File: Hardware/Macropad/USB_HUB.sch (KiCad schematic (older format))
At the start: 25 parts, among them J4 USB_C_Receptacle_USB2.0, J5 USB_C_Receptacle_USB2.0, J6 USB_C_Receptacle_USB2.0, U4 TUSB2046b, U6 SRV05-4, U8 SRV05-4, X2 625L3C006M00000

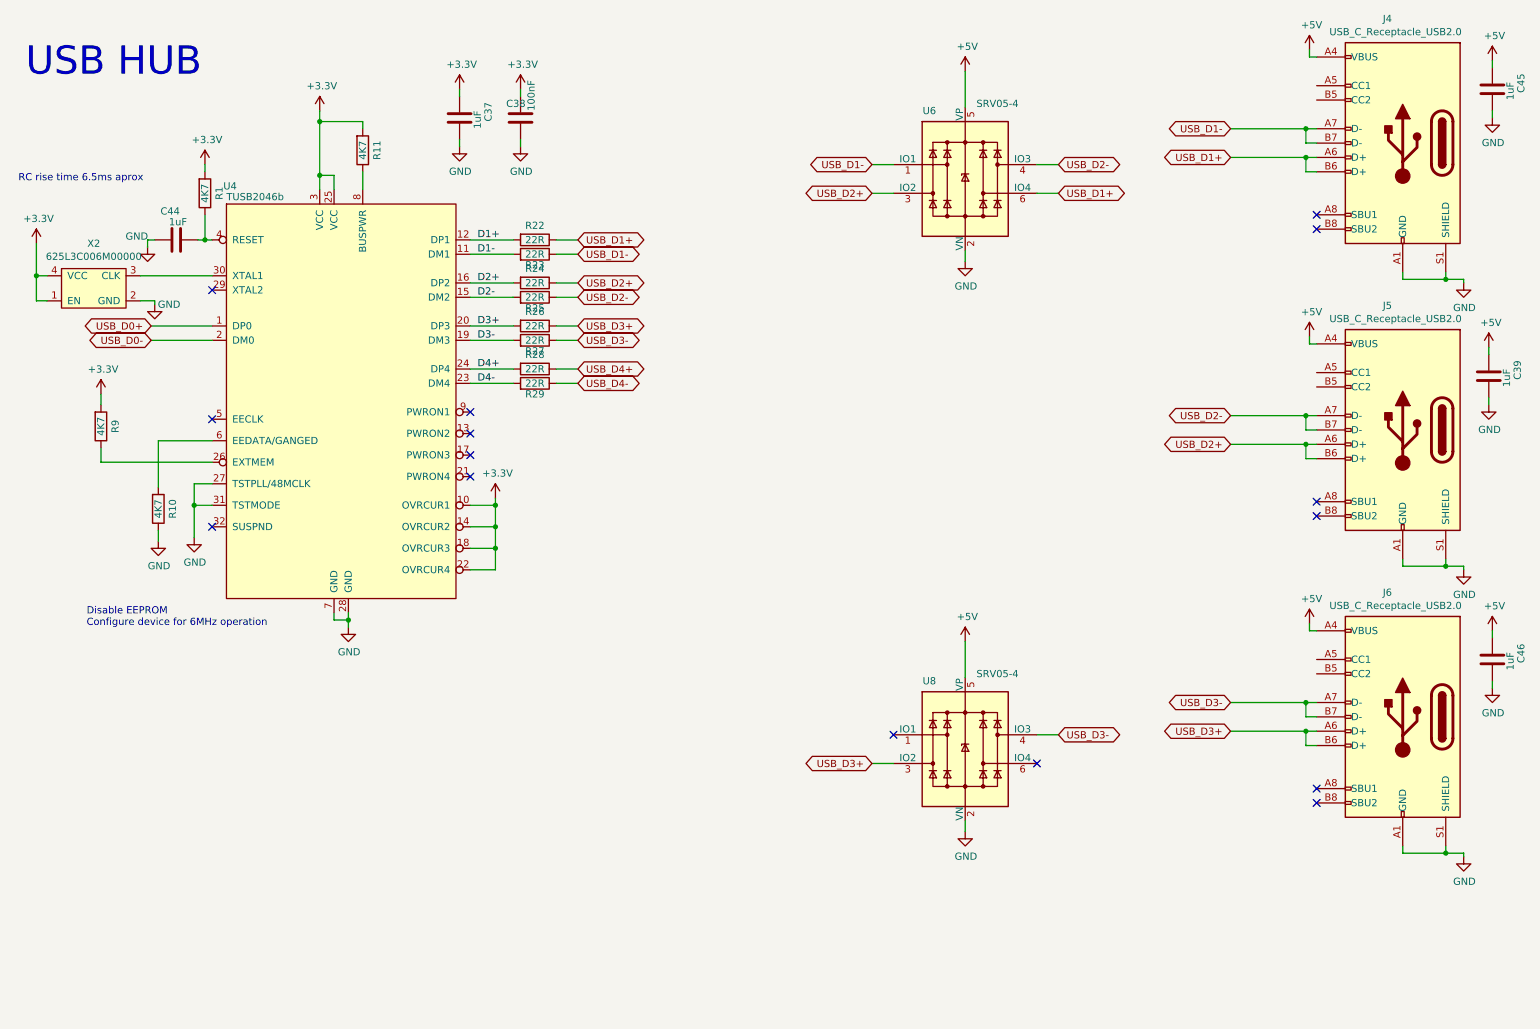
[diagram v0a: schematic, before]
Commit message: Layout done, cleaned up schematic and generated gerbers
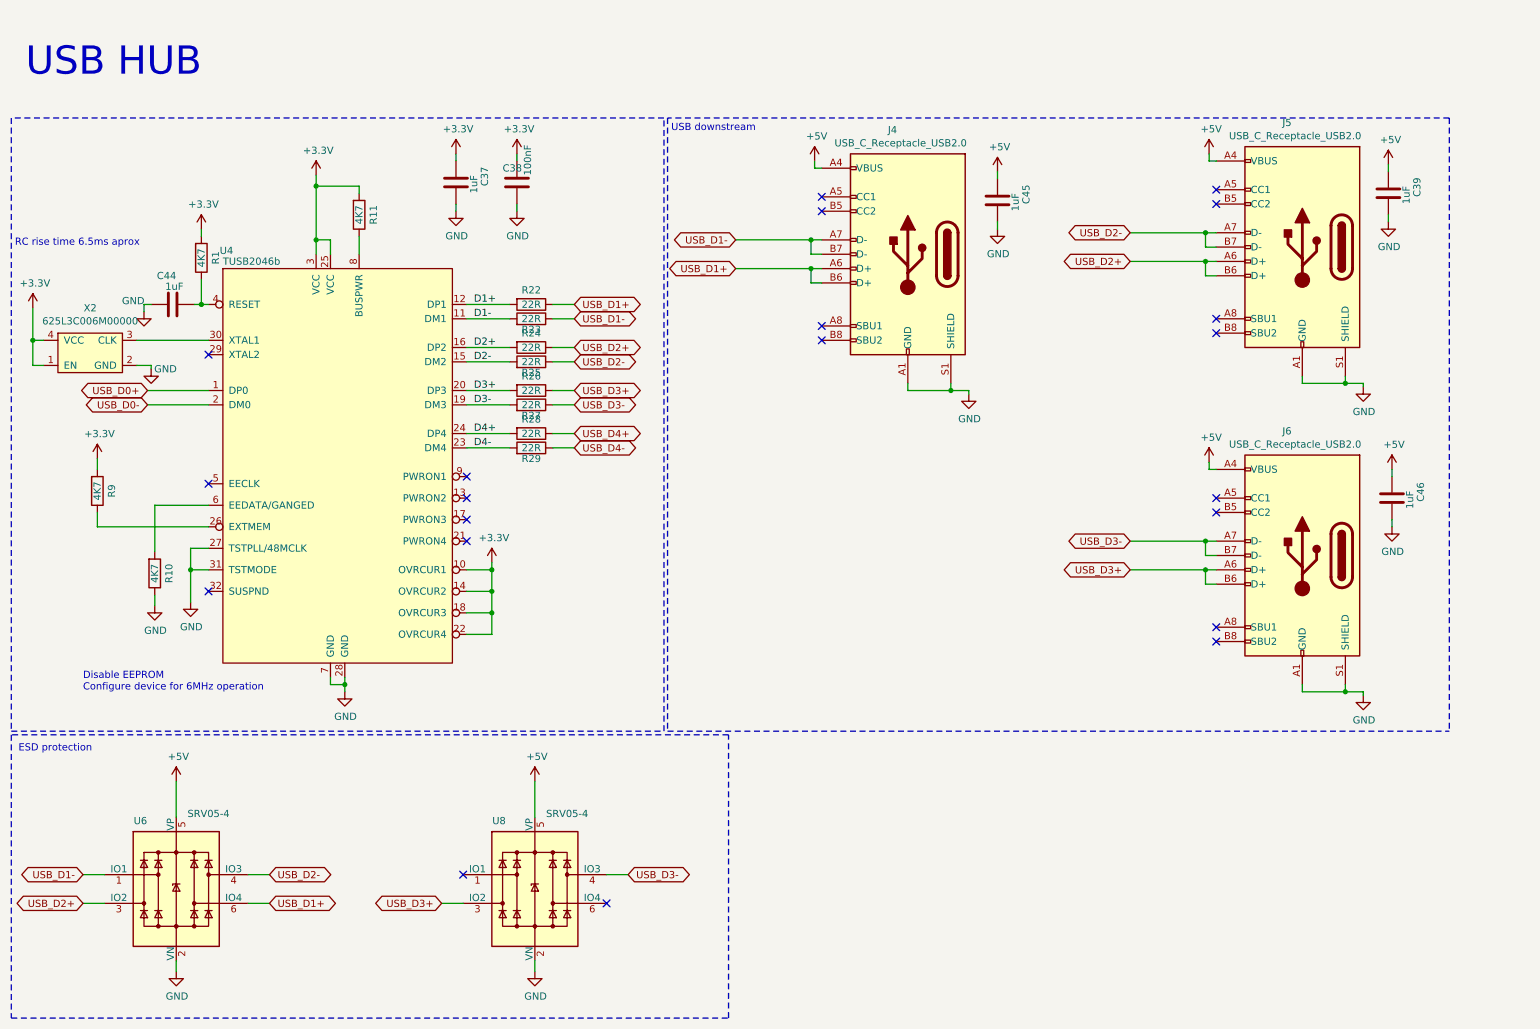
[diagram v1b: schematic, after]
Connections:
- no-connect marks 15 -> 21
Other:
- note added: "ESD protection"
- note added: "USB downstream"
- moved on the sheet: C37, C38, C39, C44, C45, C46, J4, J5, J6, R1, R10, R11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
